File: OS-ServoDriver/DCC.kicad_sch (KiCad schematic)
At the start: 5 parts, among them U701 6N137

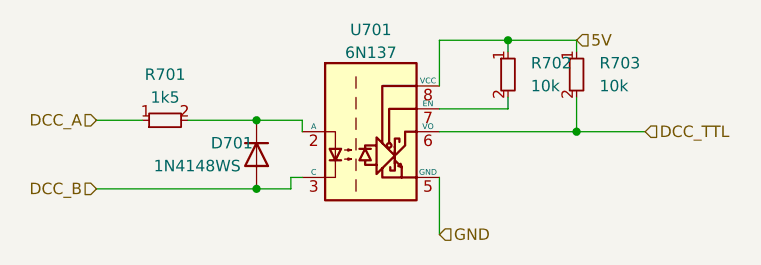
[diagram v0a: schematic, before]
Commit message: commit 4 push
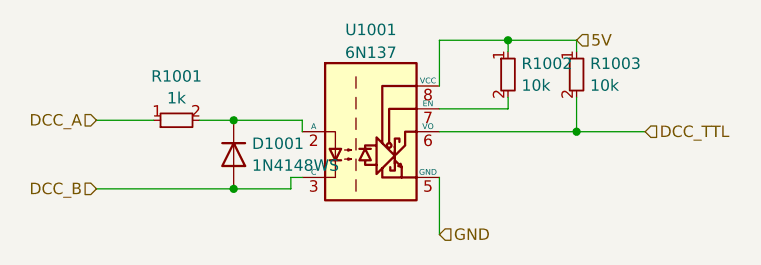
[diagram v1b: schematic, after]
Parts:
- removed D701: 1N4148WS, Diode_SMD:D_SOD-323, symbol custom_kicad_lib_sk:1N4148WS
- removed R701: 1k5, custom_kicad_lib_sk:R_0603_smalltext, symbol resistors_0603:R_1k5_0603
- removed R702, R703: 10k, custom_kicad_lib_sk:R_0603_smalltext, symbol resistors_0603:R_10k_0603
- added D1001: 1N4148WS, Diode_SMD:D_SOD-323, symbol custom_kicad_lib_sk:1N4148WS
- added R1001: 1k, custom_kicad_lib_sk:R_0603_smalltext, symbol resistors_0603:R_1k_0603
- added R1002, R1003: 10k, custom_kicad_lib_sk:R_0603_smalltext, symbol resistors_0603:R_10k_0603
- renumbered U701 to U1001
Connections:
- net 5V: now also R1002.1, R1003.1
- net DCC_A: now also R1001.1
- net DCC_B: now also D1001.2 (A)
- net DCC_TTL: now also R1003.2
- net at U1001.7 (EN): now also R1002.2
- net at U1001.2 (A): now also D1001.1 (K), R1001.2
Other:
- company: Train-Science -> (none)
